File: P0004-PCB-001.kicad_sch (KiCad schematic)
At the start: 24 parts, among them CN1 Molex 105057-0001, CN2 104031-0811, CN3 Liansheng PH--00603, SW1 Khon TSA06131-100B332CA, SW2 Khon TSA06131-100B332CA, SW3 Khon TSA06131-100B332CA, SW4 Khon TSA06131-100B332CA

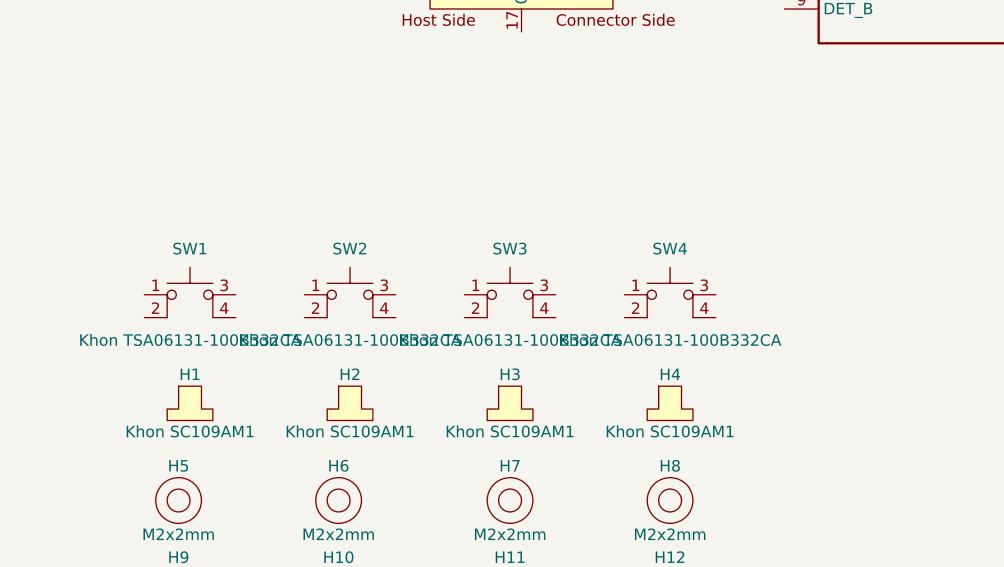
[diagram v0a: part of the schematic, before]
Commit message: testing ci config
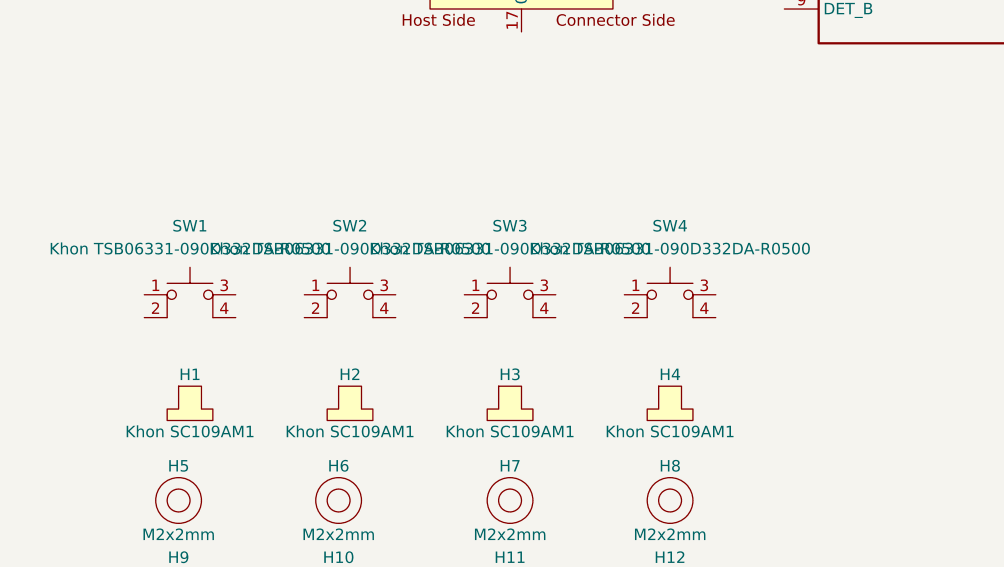
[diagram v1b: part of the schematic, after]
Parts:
- SW1, SW2, SW3, SW4: value Khon TSA06131-100B332CA -> Khon TSB06331-090D332DA-R0500
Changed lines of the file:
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@@
 		(fields_autoplaced yes)
 		(property "Reference" "SW2"
+			(at 78.74 88.9 0)
+			(show_name no)
+			(do_not_autoplace no)
+			(effects
+				(font
+					(size 1.27 1.27)
+				)
+			)
+		)
+		(property "Value" "Khon TSB06331-090D332DA-R0500"
 			(at 78.74 91.44 0)
 			(show_name no)
 			(do_not_autoplace no)
-			(effects
-				(font
-					(size 1.27 1.27)
-				)
-			)
-		)
-		(property "Value" "Khon TSA06131-100B332CA"
-			(at 78.74 101.6 0)
-			(show_name no)
-			(do_not_autoplace yes)
 			(effects
 				(font
@@
 		(fields_autoplaced yes)
 		(property "Reference" "SW4"
+			(at 114.3 88.9 0)
+			(show_name no)
+			(do_not_autoplace no)
+			(effects
+				(font
+					(size 1.27 1.27)
+				)
+			)
+		)
+		(property "Value" "Khon TSB06331-090D332DA-R0500"
 			(at 114.3 91.44 0)
 			(show_name no)
 			(do_not_autoplace no)
-			(effects
-				(font
-					(size 1.27 1.27)
-				)
-			)
-		)
-		(property "Value" "Khon TSA06131-100B332CA"
-			(at 114.3 101.6 0)
-			(show_name no)
-			(do_not_autoplace yes)
 			(effects
 				(font
@@
 		(in_bom yes)
 		(on_board yes)
-		(in_pos_files yes)
+		(in_pos_files no)
 		(dnp no)
 		(fields_autoplaced yes)
@@
 		(in_bom yes)
 		(on_board yes)
-		(in_pos_files yes)
+		(in_pos_files no)
 		(dnp no)
 		(fields_autoplaced yes)
@@
 		(fields_autoplaced yes)
 		(property "Reference" "SW1"
+			(at 60.96 88.9 0)
+			(show_name no)
+			(do_not_autoplace no)
+			(effects
+				(font
+					(size 1.27 1.27)
+				)
+			)
+		)
+		(property "Value" "Khon TSB06331-090D332DA-R0500"
 			(at 60.96 91.44 0)
 			(show_name no)
 			(do_not_autoplace no)
-			(effects
-				(font
-					(size 1.27 1.27)
-				)
-			)
-		)
-		(property "Value" "Khon TSA06131-100B332CA"
-			(at 60.96 101.6 0)
-			(show_name no)
-			(do_not_autoplace yes)
 			(effects
 				(font
@@
 		(in_bom yes)
 		(on_board yes)
-		(in_pos_files yes)
+		(in_pos_files no)
 		(dnp no)
 		(fields_autoplaced yes)
@@
 		(fields_autoplaced yes)
 		(property "Reference" "SW3"
+			(at 96.52 88.9 0)
+			(show_name no)
+			(do_not_autoplace no)
+			(effects
+				(font
+					(size 1.27 1.27)
+				)
+			)
+		)
+		(property "Value" "Khon TSB06331-090D332DA-R0500"
 			(at 96.52 91.44 0)
 			(show_name no)
 			(do_not_autoplace no)
-			(effects
-				(font
-					(size 1.27 1.27)
-				)
-			)
-		)
-		(property "Value" "Khon TSA06131-100B332CA"
-			(at 96.52 101.6 0)
-			(show_name no)
-			(do_not_autoplace yes)
 			(effects
 				(font
@@
 		(in_bom yes)
 		(on_board yes)
-		(in_pos_files yes)
+		(in_pos_files no)
 		(dnp no)
 		(fields_autoplaced yes)
